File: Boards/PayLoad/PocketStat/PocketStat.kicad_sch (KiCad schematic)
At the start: 71 parts, among them J20 DX07S016JA1R1500, J3 MEM2061-01-188-00-A_REVA, J5 BM03B-SRSS-TBLFSN, Q1 BC857CMB_315, U1 HDC2080DMBR, U4 LPS22DFTR, U5 W25Q128JVSIQ TR, U6 BMP581, U8 ST1L05APU33R

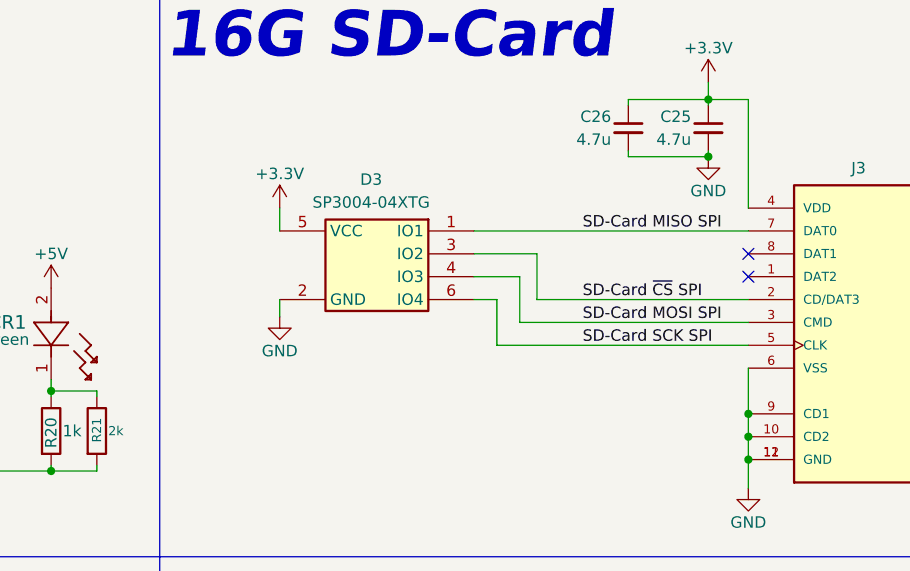
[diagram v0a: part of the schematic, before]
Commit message: PocketStat update
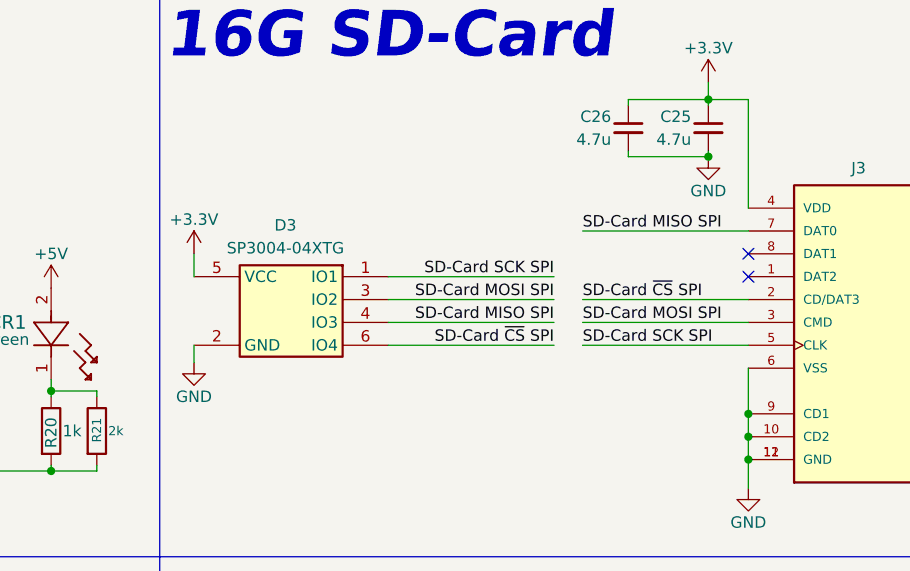
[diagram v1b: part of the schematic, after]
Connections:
- net SD-Card  ~{CS} SPI: now also D3.6 (IO4); no longer D3.3 (IO2)
- net SD-Card MISO SPI: now also D3.4 (IO3); no longer D3.1 (IO1)
- net SD-Card MOSI SPI: now also D3.3 (IO2); no longer D3.4 (IO3)
- net SD-Card SCK SPI: now also D3.1 (IO1); no longer D3.6 (IO4)
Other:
- moved on the sheet: D3
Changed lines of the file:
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@@
 	(wire
 		(pts
+			(xy 165.735 144.78) (xy 184.15 144.78)
+		)
+		(stroke
+			(width 0)
+			(type default)
+		)
+	)
+	(wire
+		(pts
 			(xy 74.93 48.895) (xy 77.47 48.895)
 		)
@@
 	(wire
 		(pts
+			(xy 165.735 147.32) (xy 184.15 147.32)
+		)
+		(stroke
+			(width 0)
+			(type default)
+		)
+	)
+	(wire
+		(pts
 			(xy 225.425 247.65) (xy 227.965 247.65)
 		)
@@
 	(wire
 		(pts
-			(xy 177.8 142.24) (xy 177.8 147.32)
+			(xy 165.735 142.24) (xy 184.15 142.24)
 		)
 		(stroke
@@
 	(wire
 		(pts
-			(xy 180.34 144.78) (xy 205.74 144.78)
+			(xy 150.495 250.19) (xy 150.495 251.46)
 		)
 		(stroke
@@
 	(wire
 		(pts
-			(xy 150.495 250.19) (xy 150.495 251.46)
+			(xy 40.64 112.395) (xy 46.99 112.395)
 		)
 		(stroke
@@
 	(wire
 		(pts
-			(xy 40.64 112.395) (xy 46.99 112.395)
+			(xy 201.295 126.365) (xy 201.295 125.73)
 		)
 		(stroke
@@
 	(wire
 		(pts
-			(xy 201.295 126.365) (xy 201.295 125.73)
+			(xy 187.325 142.24) (xy 205.74 142.24)
 		)
 		(stroke
@@
 	(wire
 		(pts
-			(xy 175.26 139.7) (xy 180.34 139.7)
-		)
-		(stroke
-			(width 0)
-			(type default)
-		)
-	)
-	(wire
-		(pts
 			(xy 265.43 223.52) (xy 266.7 223.52)
 		)
@@
 	(wire
 		(pts
-			(xy 153.67 142.24) (xy 153.67 144.145)
-		)
-		(stroke
-			(width 0)
-			(type default)
-		)
-	)
-	(wire
-		(pts
-			(xy 182.245 137.16) (xy 182.245 142.24)
+			(xy 144.145 147.32) (xy 144.145 149.225)
 		)
 		(stroke
@@
 	(wire
 		(pts
-			(xy 182.245 142.24) (xy 205.74 142.24)
-		)
-		(stroke
-			(width 0)
-			(type default)
-		)
-	)
-	(wire
-		(pts
 			(xy 171.45 36.195) (xy 171.45 43.815)
 		)
@@
 	(wire
 		(pts
+			(xy 187.325 147.32) (xy 205.74 147.32)
+		)
+		(stroke
+			(width 0)
+			(type default)
+		)
+	)
+	(wire
+		(pts
 			(xy 57.15 36.195) (xy 64.77 36.195)
 		)
@@
 	(wire
 		(pts
-			(xy 180.34 139.7) (xy 180.34 144.78)
-		)
-		(stroke
-			(width 0)
-			(type default)
-		)
-	)
-	(wire
-		(pts
 			(xy 92.71 28.575) (xy 85.09 28.575)
 		)
@@
 	(wire
 		(pts
-			(xy 175.26 137.16) (xy 182.245 137.16)
-		)
-		(stroke
-			(width 0)
-			(type default)
-		)
-	)
-	(wire
-		(pts
 			(xy 44.45 38.1) (xy 44.45 46.355)
 		)
@@
 	(wire
 		(pts
+			(xy 187.325 134.62) (xy 205.74 134.62)
+		)
+		(stroke
+			(width 0)
+			(type default)
+		)
+	)
+	(wire
+		(pts
 			(xy 97.79 125.095) (xy 116.205 125.095)
 		)
@@
 	(wire
 		(pts
-			(xy 175.26 142.24) (xy 177.8 142.24)
-		)
-		(stroke
-			(width 0)
-			(type default)
-		)
-	)
-	(wire
-		(pts
 			(xy 155.575 205.105) (xy 155.575 206.375)
 		)
@@
 	(wire
 		(pts
-			(xy 175.26 134.62) (xy 205.74 134.62)
-		)
-		(stroke
-			(width 0)
-			(type default)
-		)
-	)
-	(wire
-		(pts
 			(xy 133.35 160.655) (xy 133.35 161.29)
 		)
@@
 	(wire
 		(pts
-			(xy 153.67 132.08) (xy 153.67 134.62)
+			(xy 144.145 137.16) (xy 144.145 139.7)
 		)
 		(stroke
@@
 	(wire
 		(pts
-			(xy 177.8 147.32) (xy 205.74 147.32)
+			(xy 300.355 212.09) (xy 300.355 214.63)
 		)
 		(stroke
@@
 	(wire
 		(pts
-			(xy 300.355 212.09) (xy 300.355 214.63)
+			(xy 120.65 231.14) (xy 135.89 231.14)
 		)
 		(stroke
@@
 	(wire
 		(pts
-			(xy 120.65 231.14) (xy 135.89 231.14)
+			(xy 220.345 46.355) (xy 220.345 43.815)
 		)
 		(stroke
@@
 		)
 	)
-	(wire
+	(polyline
 		(pts
-			(xy 220.345 46.355) (xy 220.345 43.815)
+			(xy 235.585 104.775) (xy 235.585 248.285)
 		)
 		(stroke
@@
 		)
 	)
-	(polyline
+	(wire
 		(pts
-			(xy 235.585 104.775) (xy 235.585 248.285)
+			(xy 230.505 43.815) (xy 230.505 45.085)
 		)
 		(stroke
@@
 	(wire
 		(pts
-			(xy 230.505 43.815) (xy 230.505 45.085)
+			(xy 165.735 139.7) (xy 184.15 139.7)
 		)
 		(stroke
@@
 	(wire
 		(pts
+			(xy 187.325 144.78) (xy 205.74 144.78)
+		)
+		(stroke
+			(width 0)
+			(type default)
+		)
+	)
+	(wire
+		(pts
 			(xy 149.86 36.195) (xy 149.86 40.64)
 		)
@@
 		)
 	)
+	(label "SD-Card SCK SPI"
+		(at 184.15 139.7 180)
+		(effects
+			(font
+				(size 1.27 1.27)
+			)
+			(justify right bottom)
+		)
+	)
 	(label "SCL0 I2C"
 		(at 116.205 120.015 180)
@@
 		)
 	)
+	(label "SD-Card MOSI SPI"
+		(at 184.15 142.24 180)
+		(effects
+			(font
+				(size 1.27 1.27)
+			)
+			(justify right bottom)
+		)
+	)
 	(label "MOSI1 SPI"
 		(at 116.205 84.455 180)
@@
 	)
 	(label "SD-Card MISO SPI"
+		(at 184.15 144.78 180)
+		(effects
+			(font
+				(size 1.27 1.27)
+			)
+			(justify right bottom)
+		)
+	)
+	(label "SD-Card MISO SPI"
 		(at 187.325 134.62 0)
 		(effects
@@
 		)
 	)
+	(label "SD-Card  ~{CS} SPI"
+		(at 184.15 147.32 180)
+		(effects
+			(font
+				(size 1.27 1.27)
+			)
+			(justify right bottom)
+		)
+	)
 	(label "MCU SCLK SPI"
 		(at 31.75 89.535 0)
@@
 	(symbol
 		(lib_id "power:GND")
-		(at 153.67 144.145 0)
+		(at 144.145 149.225 0)
 		(unit 1)
 		(exclude_from_sim no)
@@
 		(dnp no)
 		(property "Reference" "#PWR018"
-			(at 153.67 150.495 0)
+			(at 144.145 155.575 0)
 			(effects
 				(font
@@
 		)
 		(property "Value" "GND"
-			(at 153.67 147.955 0)
+			(at 144.145 153.035 0)
 			(effects
 				(font
@@
 		)
 		(property "Footprint" ""
-			(at 153.67 144.145 0)
+			(at 144.145 149.225 0)
 			(effects
 				(font
@@
 		)
 		(property "Datasheet" ""
-			(at 153.67 144.145 0)
+			(at 144.145 149.225 0)
 			(effects
 				(font
@@
 		)
 		(property "Description" "Power symbol creates a global label with name \"GND\" , ground"
-			(at 153.67 144.145 0)
+			(at 144.145 149.225 0)
 			(effects
 				(font
@@
 	(symbol
 		(lib_id "power:+3.3V")
-		(at 153.67 132.08 0)
+		(at 144.145 137.16 0)
 		(unit 1)
 		(exclude_from_sim no)
@@
 		(dnp no)
 		(property "Reference" "#PWR017"
-			(at 153.67 135.89 0)
+			(at 144.145 140.97 0)
 			(effects
 				(font
@@
 		)
 		(property "Value" "+3.3V"
-			(at 153.67 128.27 0)
+			(at 144.145 133.35 0)
 			(effects
 				(font
@@
 		)
 		(property "Footprint" ""
-			(at 153.67 132.08 0)
+			(at 144.145 137.16 0)
 			(effects
 				(font
@@
 		)
 		(property "Datasheet" ""
-			(at 153.67 132.08 0)
+			(at 144.145 137.16 0)
 			(effects
 				(font
@@
 		)
 		(property "Description" "Power symbol creates a global label with name \"+3.3V\""
-			(at 153.67 132.08 0)
+			(at 144.145 137.16 0)
 			(effects
 				(font
@@
 	(symbol
 		(lib_id "SP3004-04XTG:SP3004-04XTG")
-		(at 175.26 134.62 0)
+		(at 165.735 139.7 0)
 		(mirror y)
 		(unit 1)
@@
 		(dnp no)
 		(property "Reference" "D3"
-			(at 163.83 128.905 0)
+			(at 154.305 133.985 0)
 			(effects
 				(font
@@
 		)
 		(property "Value" "SP3004-04XTG"
-			(at 163.83 131.445 0)
+			(at 154.305 136.525 0)
 			(effects
 				(font
@@
 		)
 		(property "Footprint" "TVS-SP3004:SOT563_LTF"
-			(at 148.59 229.54 0)
+			(at 139.065 234.62 0)
 			(effects
 				(font
@@
 		)
 		(property "Datasheet" "https://m.littelfuse.com/~/media/electronics/datasheets/tvs_diode_arrays/littelfuse_tvs_diode_array_sp3004_datasheet.pdf.pdf"
-			(at 148.59 329.54 0)
+			(at 139.065 334.62 0)
 			(effects
 				(font
@@
 		)
 		(property "Description" "LITTELFUSE - SP3004-04XTG - TVS Diode, Unidirectional, 6 V, 15 V, SOT-563, 6 Pins"
-			(at 175.26 134.62 0)
+			(at 165.735 139.7 0)
 			(effects
 				(font
@@
 		)
 		(property "Height" "0.6"
-			(at 148.59 529.54 0)
+			(at 139.065 534.62 0)
 			(effects
 				(font
@@
 		)
 		(property "Mouser Part Number" "576-SP3004-04XTG"
-			(at 148.59 629.54 0)
+			(at 139.065 634.62 0)
 			(effects
 				(font
@@
 		)
 		(property "Mouser Price/Stock" "https://www.mouser.co.uk/ProductDetail/Littelfuse/SP3004-04XTG?qs=trbuaetfxXQ7JjseAkJ3Ww%3D%3D"
-			(at 148.59 729.54 0)
+			(at 139.065 734.62 0)
 			(effects
 				(font
@@
 		)
 		(property "Manufacturer_Name" "LITTELFUSE"
-			(at 148.59 829.54 0)
+			(at 139.065 834.62 0)
 			(effects
 				(font
@@
 		)
 		(property "Manufacturer_Part_Number" "SP3004-04XTG"
-			(at 148.59 929.54 0)
+			(at 139.065 934.62 0)
 			(effects
 				(font
